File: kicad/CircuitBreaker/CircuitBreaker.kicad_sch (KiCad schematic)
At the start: 33 parts

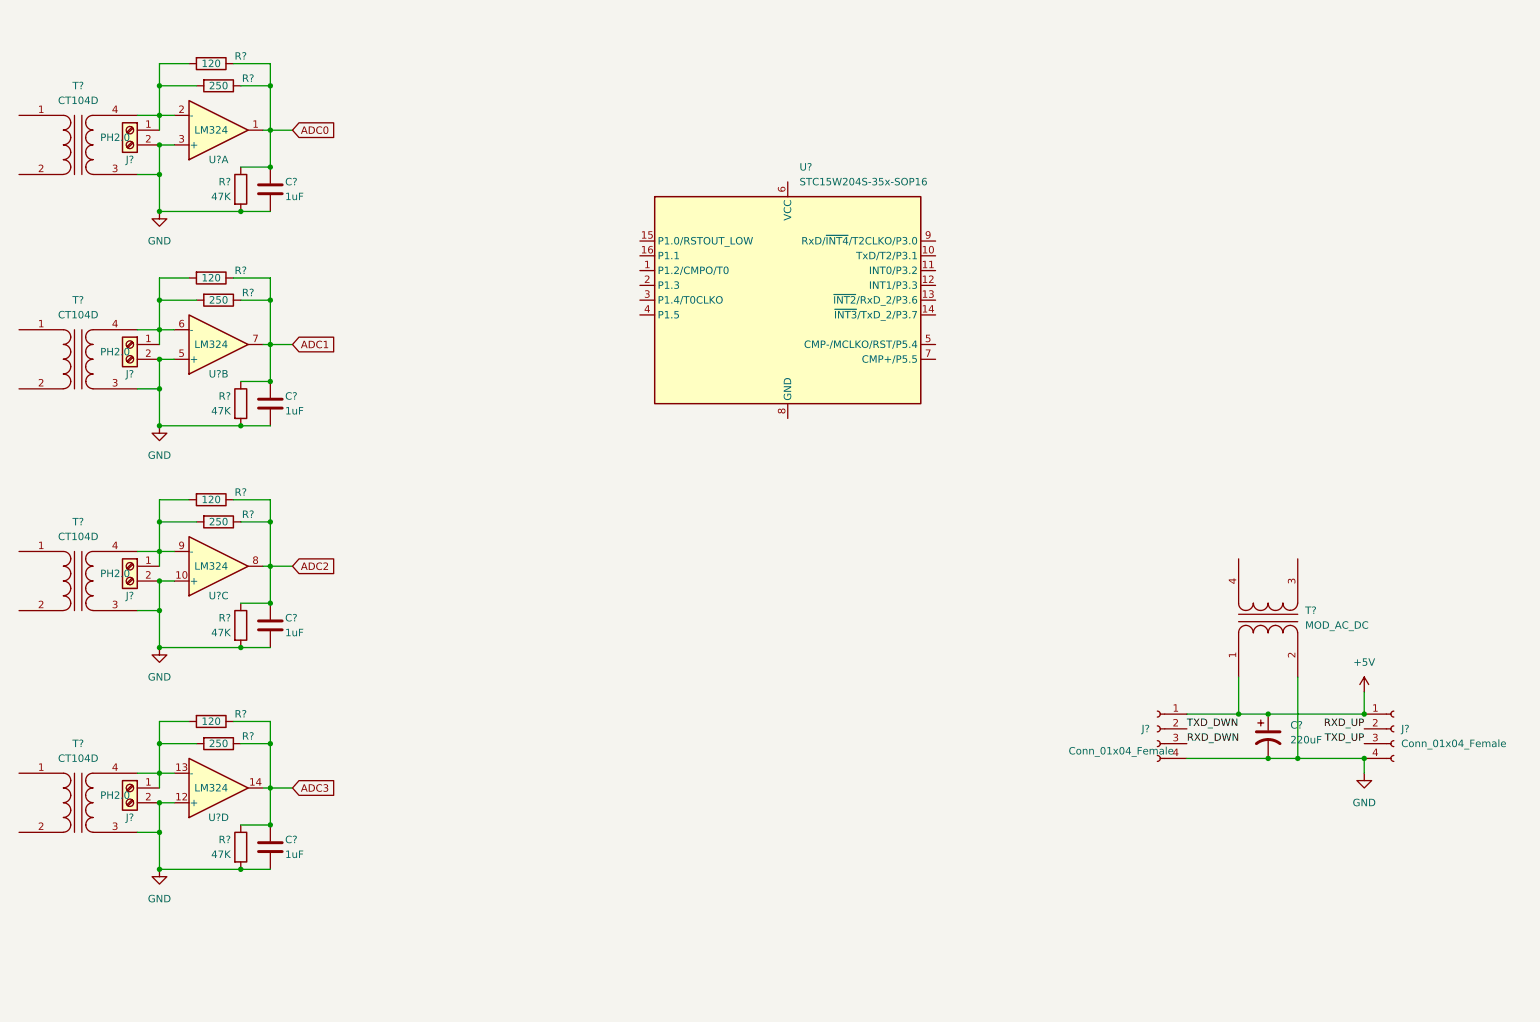
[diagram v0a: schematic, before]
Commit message: pwr and up/down link
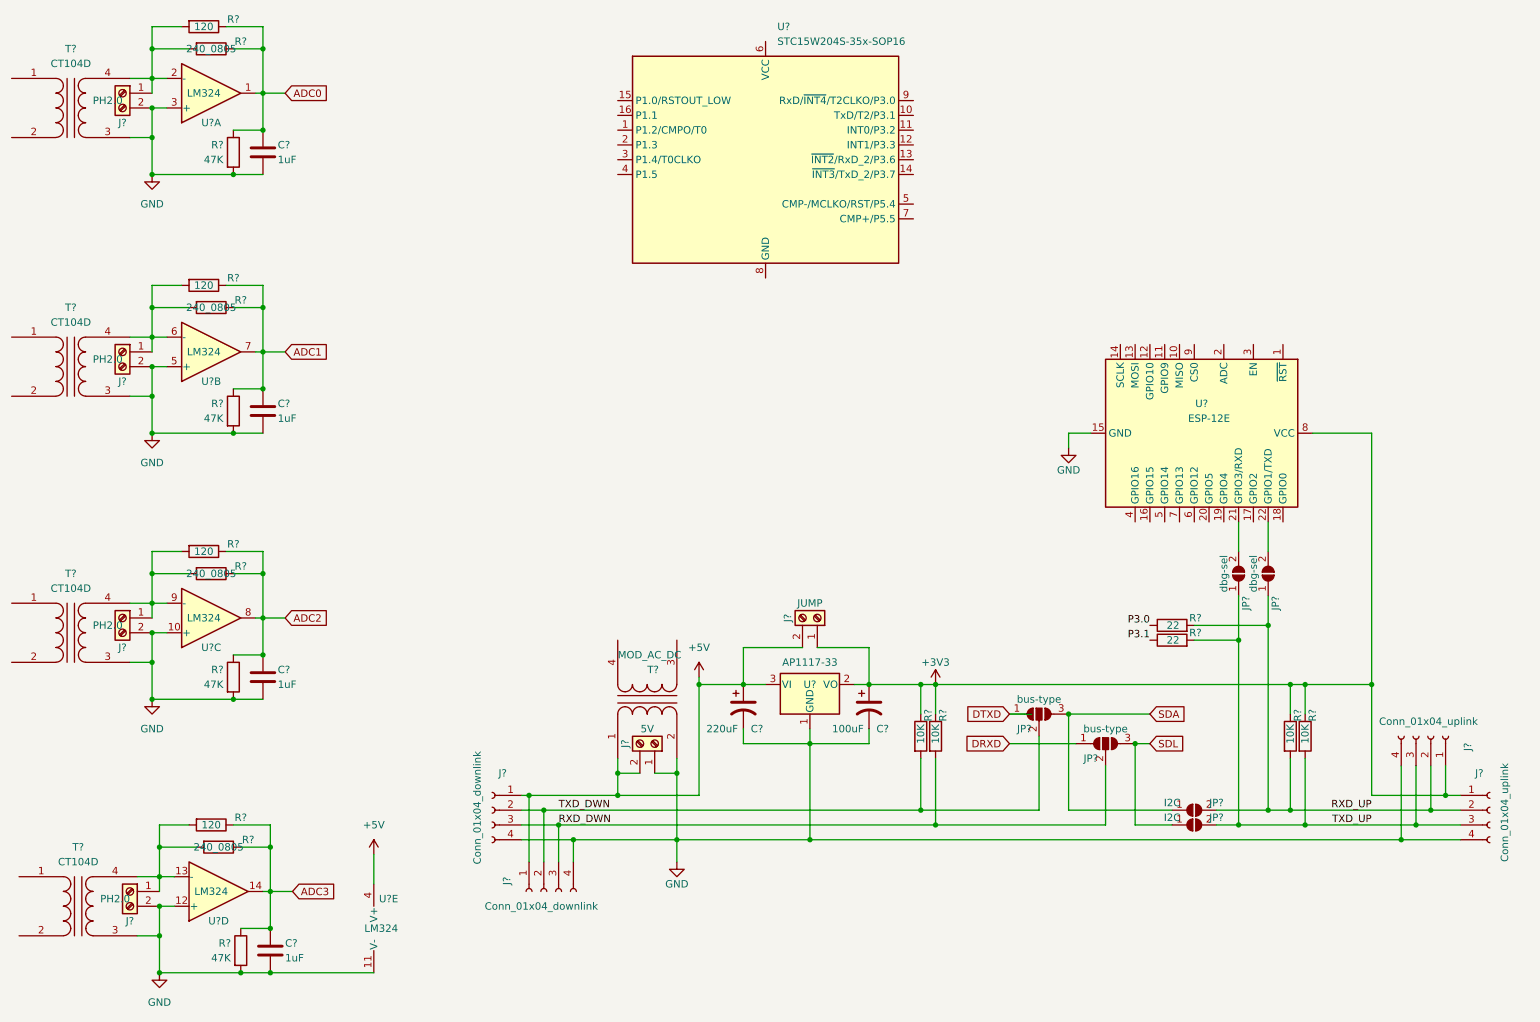
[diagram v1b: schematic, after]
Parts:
- added C?: 100uF, symbol Device:C_Polarized_US
- added J?: 5V, symbol Connector:Screw_Terminal_01x02
- added J?: Conn_01x04_downlink, symbol Connector:Conn_01x04_Female
- added J?: JUMP, symbol Connector:Screw_Terminal_01x02
- added J?: Conn_01x04_uplink, symbol Connector:Conn_01x04_Female
- added JP? (x2): I2C, symbol Jumper:SolderJumper_2_Open
- added JP? (x2): dbg-sel, symbol Jumper:SolderJumper_2_Open
- added JP? (x2): bus-type, symbol Jumper:SolderJumper_3_Open
- added R? (x4): 10K, symbol Device:R
- added R? (x2): 22, symbol Device:R
- added U?: AP1117-33, Package_TO_SOT_SMD:SOT-223-3_TabPin2, symbol Regulator_Linear:AP1117-33
- added U?: LM324, symbol Amplifier_Operational:LM324
- added U?: ESP-12E, RF_Module:ESP-12E, symbol RF_Module:ESP-12E
- J?: value Conn_01x04_Female -> Conn_01x04_uplink
- J?: value Conn_01x04_Female -> Conn_01x04_downlink
- R? (x4): value 250 -> 240_0805
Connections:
- net +5V: now also J?.1 (Pin_1), J?.2 (Pin_2), J?.2 (Pin_2), U?.3 (VI), U?.4 (V+); no longer J?.1 (Pin_1)
- net GND: now also C?.2, J?.1 (Pin_1), J?.4 (Pin_4), J?.4 (Pin_4), U?.1 (GND), U?.11 (V-), U?.15 (GND)
- net RXD_DWN: now also J?.3 (Pin_3), JP?.2 (C), R?.2
- net RXD_UP: now also J?.2 (Pin_2), JP?.1 (A), JP?.2 (B), R?.2, R?.2
- net TXD_DWN: now also J?.2 (Pin_2), JP?.2 (C), R?.2
- net TXD_UP: now also J?.3 (Pin_3), JP?.1 (A), JP?.2 (B), R?.2, R?.2
- new net: JP?.2 (B), U?.21 (GPIO3/RXD)
- new net: JP?.2 (B), U?.22 (GPIO1/TXD)
- new net +3V3: C?.1, J?.1 (Pin_1), J?.1 (Pin_1), J?.1 (Pin_1), R?.1, R?.1, R?.1, R?.1, U?.2 (VO), U?.8 (VCC)
- new net DRXD: JP?.1 (A)
- new net DTXD: JP?.1 (A)
- new net P3.0: R?.1
- new net P3.1: R?.1
- new net SDA: JP?.1 (A), JP?.3 (B)
- new net SDL: JP?.1 (A), JP?.3 (B)
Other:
- moved on the sheet: C?, J?, R?, T?, U?, U?A, U?B, U?C, U?D
